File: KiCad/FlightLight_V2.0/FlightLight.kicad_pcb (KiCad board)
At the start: 2 copper layers, 33.5 x 35.5 mm, 27 parts, among them J3 Conn_02x05_Odd_Even, SW1 AP, U2 ULN2003, U3 ESP-12F, U4 AMS1117-3.3

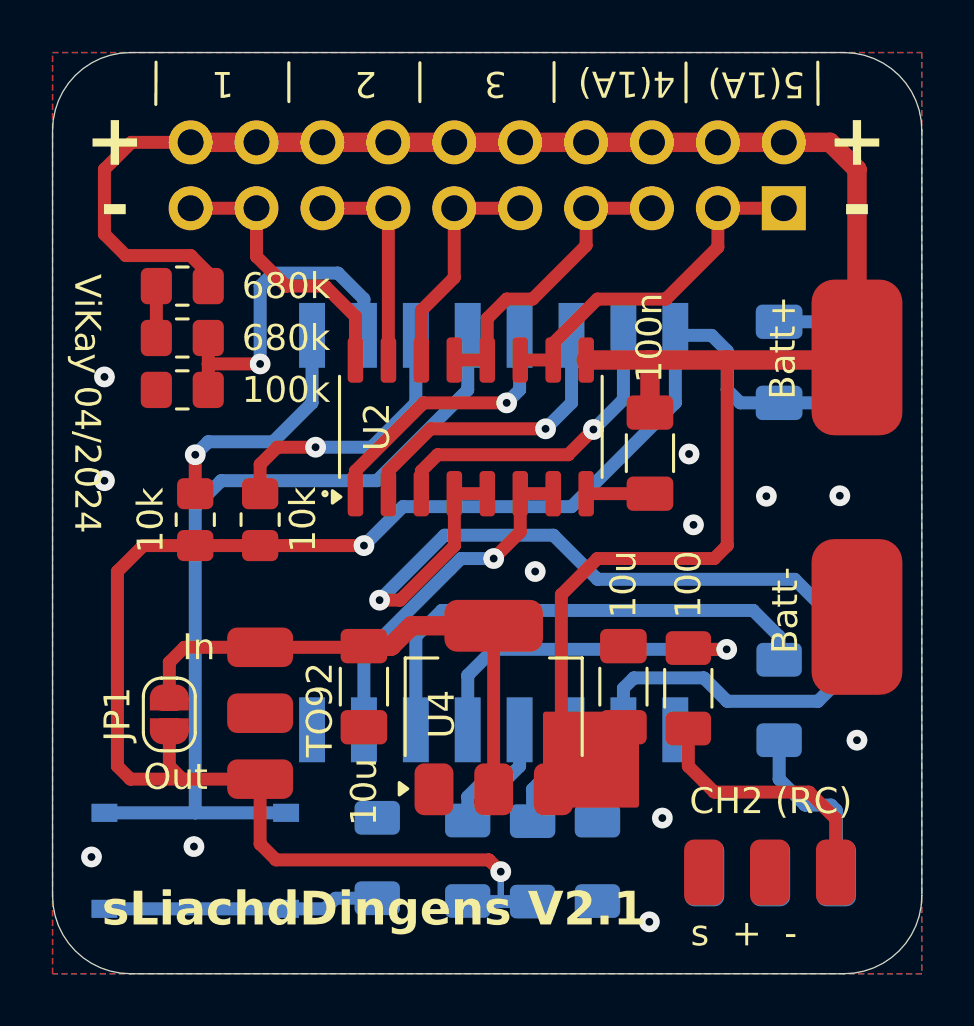
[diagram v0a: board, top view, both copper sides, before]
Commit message: PCB V2.1
kleine Fixes
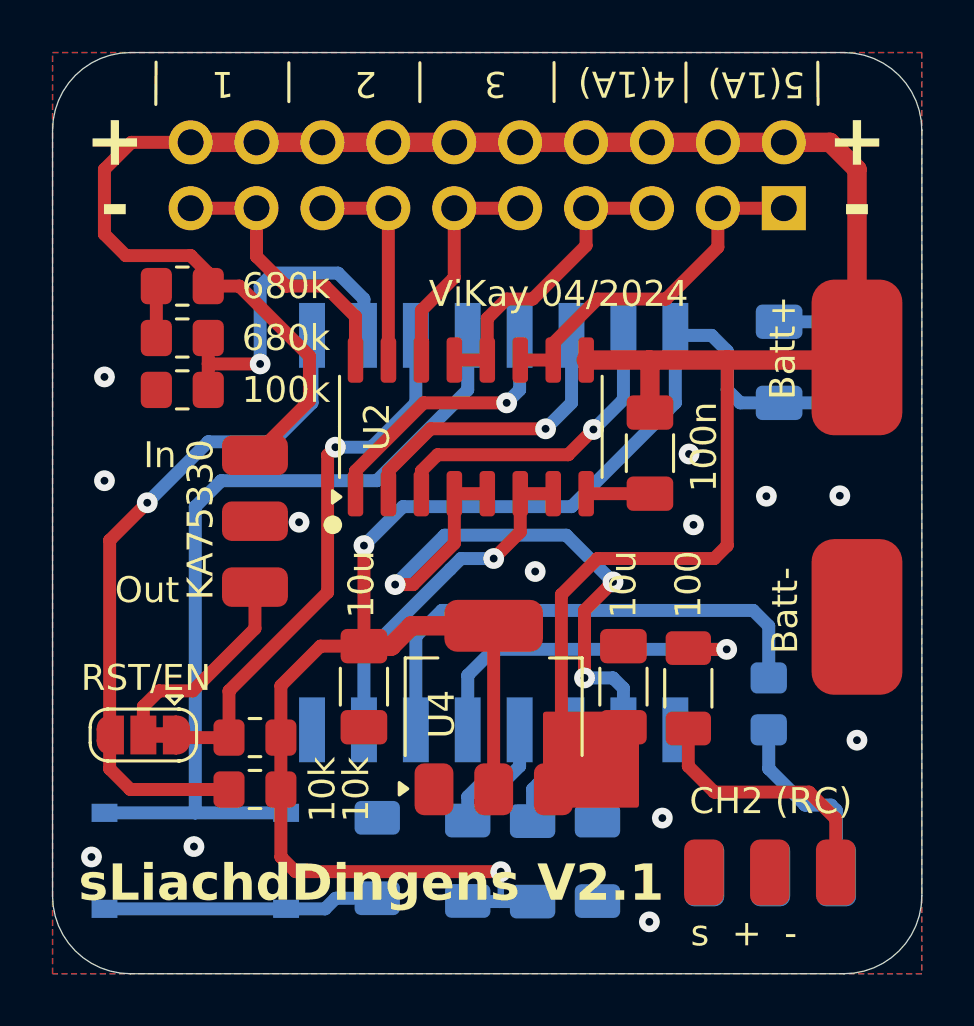
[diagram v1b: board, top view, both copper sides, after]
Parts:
- JP1: value kein Supervisor -> RST/EN; footprint Jumper:SolderJumper-2_P1.3mm_Open_RoundedPad1.0x1.5mm -> Jumper:SolderJumper-3_P1.3mm_Bridged12_RoundedPad1.0x1.5mm
- R7: footprint Resistor_SMD:R_1206_3216Metric_Pad1.30x1.75mm_HandSolder -> Resistor_SMD:R_0805_2012Metric_Pad1.20x1.40mm_HandSolder
- moved R3 10.7 mm to (109.3, 89.4), turned to 180 degrees
- moved R1 8.40 mm to (109.3, 87.4), turned to 180 degrees
- moved TO92 7.40 mm to (109.3, 76.5)
- moved JP1 1.28 mm to (105.0, 87.3), turned to 180 degrees
- moved R7 0.43 mm to (129.1, 86.1)
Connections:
- C4 pad 1: Net-(JP1-A) -> 3,3V
- JP1 pad 1: Net-(JP1-A) -> EN
- JP1 pad 2: 3,3V -> EN/RST
- R1 pad 2: Net-(U3-EN) -> EN
- R3 pad 2: Net-(U3-~{RST}) -> RST
- TO92 pad 1: Net-(JP1-A) -> +BATT
- TO92 pad 3: 3,3V -> EN/RST
- U3 pad 1: Net-(U3-~{RST}) -> RST
- U3 pad 3: Net-(U3-EN) -> EN
- U4 pad 2: Net-(JP1-A) -> 3,3V
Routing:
- net RST: track 0.00 -> 26.3 mm, vias 0 -> 1
- net EN: track 0.00 -> 21.5 mm, vias 0 -> 1
- net Net-(JP1-A): track 20.7 -> 0.00 mm
- net D8: track 44.1 -> 27.5 mm, vias 1 -> 3
- net Net-(U3-EN): track 10.7 -> 0.00 mm, vias 1 -> 0
- net +BATT: track 83.6 -> 93.3 mm
- net Net-(U3-~{RST}): track 9.43 -> 0.00 mm, vias 1 -> 0
- net EN/RST: track 0.00 -> 8.24 mm
- net 3,3V: track 66.5 -> 63.8 mm
- net /CH1: track 6.63 -> 7.20 mm
- net D1: track 19.3 -> 19.9 mm
- net -BATT: vias 12 -> 13
